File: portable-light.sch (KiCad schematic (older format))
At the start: 97 parts, among them J1 Conn_01x08, J2 Prog, Q1 MMBT2222A, Q2 MMBT2222A, Q3 MMBT2222A, Q4 MMBT2222A, Q5 MMBT2222A, Q6 PHD45N03LTA, Q7 PHD45N03LTA, Q8 MMBT2222A, U1 ATmega88PA-AU, U2 L78L05_SOT89, U3 LTC1733EMSEPBF, X1 LOAD, Y1 Crystal

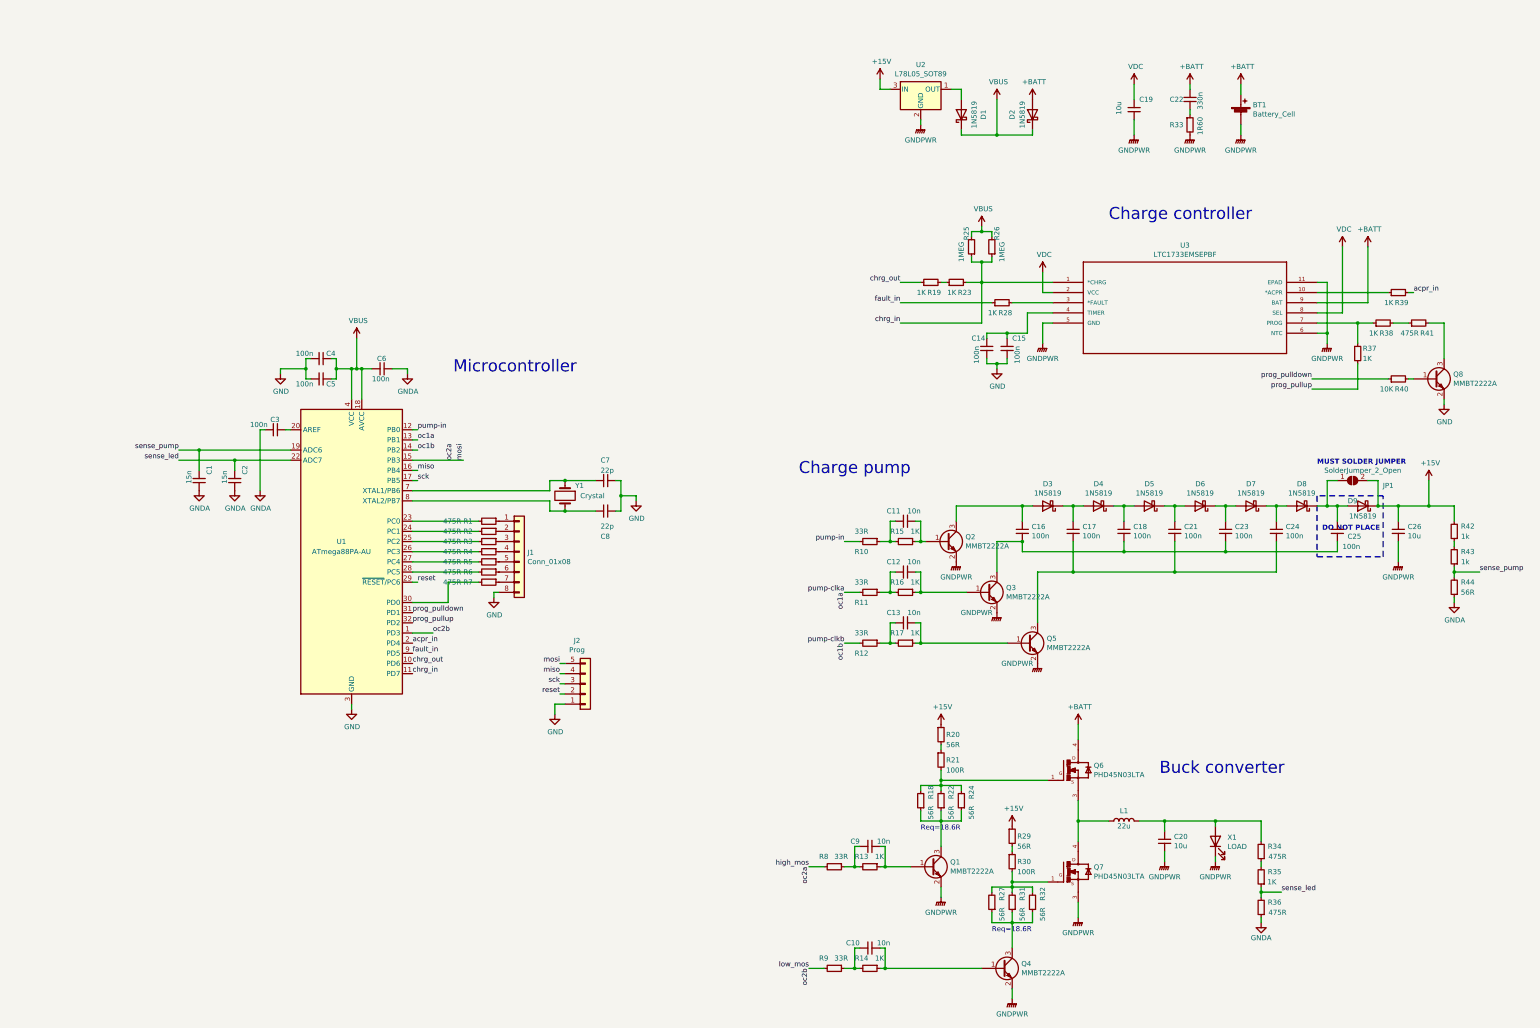
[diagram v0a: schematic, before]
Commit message: Schematics and PCB layout complete
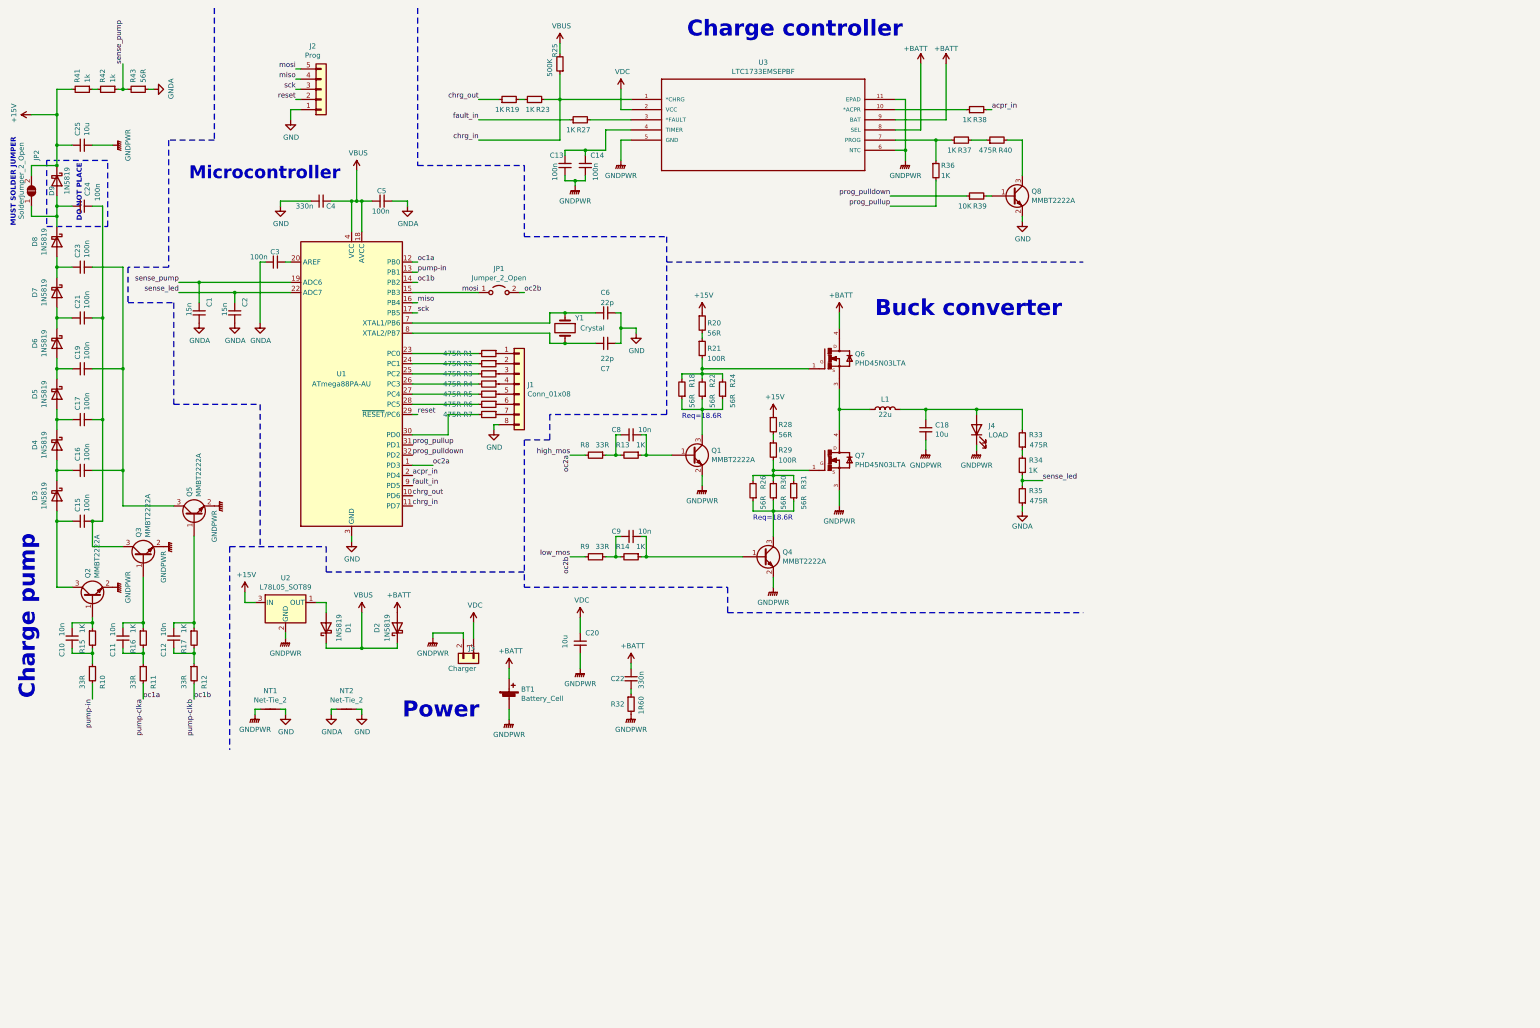
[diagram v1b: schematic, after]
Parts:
- removed C4: 100n, Capacitor_SMD:C_1206_3216Metric_Pad1.42x1.75mm_HandSolder, symbol Device:C_Small
- removed R26: 1MEG, Resistor_THT:R_Axial_DIN0309_L9.0mm_D3.2mm_P12.70mm_Horizontal, symbol Device:R_Small
- added J3: Charger, Connector_PinHeader_2.54mm:PinHeader_1x02_P2.54mm_Vertical, symbol Connector_Generic:Conn_01x02
- added JP1: Jumper_2_Open, Jumper:SolderJumper-2_P1.3mm_Open_RoundedPad1.0x1.5mm, symbol Jumper:Jumper_2_Open
- added NT1, NT2: Net-Tie_2, NetTie:NetTie-2_SMD_Pad0.5mm, symbol Device:Net-Tie_2
- BT1: footprint Connector_PinHeader_1.00mm:PinHeader_1x02_P1.00mm_Vertical -> Connector_PinHeader_2.54mm:PinHeader_1x02_P2.54mm_Vertical
- C4: renamed from C5; value 100n -> 330n
- R25: value 1MEG -> 500K
- renumbered C11 to C10, C12 to C11, C13 to C12, C14 to C13, C15 to C14, C16 to C15, C17 to C16, C18 to C17, C20 to C18, C21 to C19, C19 to C20, C23 to C21, C24 to C23, C25 to C24, C26 to C25, C6 to C5, C7 to C6, C8 to C7, C9 to C8, C10 to C9, X1 to J4, JP1 to JP2, R27 to R26, R28 to R27, R29 to R28, R30 to R29, R31 to R30, R32 to R31, R33 to R32, R34 to R33, R35 to R34, R36 to R35, R37 to R36, R38 to R37, R39 to R38, R40 to R39, R41 to R40, R42 to R41, R43 to R42, R44 to R43
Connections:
- net +BATT: now also U3.8 (SEL)
- net GND: now also NT1.1, NT2.1; no longer C13.2, C14.2
- net GNDA: now also NT2.2
- net GNDPWR: now also C13.2, C14.2, J3.2 (Pin_2), NT1.2
- net VDC: now also J3.1 (Pin_1); no longer U3.8 (SEL)
- net high_mos: now also U1.1 (PD3); no longer J2.5 (Pin_5), U1.15 (PB3)
- net low_mos: now also JP1.2 (B); no longer U1.1 (PD3)
- net oc1a: now also U1.12 (PB0); no longer U1.13 (PB1)
- net prog_pulldown: now also U1.32 (PD2); no longer U1.31 (PD1)
- net prog_pullup: now also U1.31 (PD1); no longer U1.32 (PD2)
- net pump-in: now also U1.13 (PB1); no longer U1.12 (PB0)
- new net mosi: J2.5 (Pin_5), JP1.1 (A), U1.15 (PB3)
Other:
- note added: "Power"
- moved on the sheet: BT1, C1, C10, C11, C12, C13, C14, C15, C16, C17, C18, C19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
